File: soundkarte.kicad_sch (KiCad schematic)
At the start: 76 parts, among them J1 Data, J10 Address, J2 Control, J3 Bus Blaster, J4 Power, J5 1-28, J6 JTAG, J7 29-56, J8 Main Power, J9 Aux Power, U1 Teensy++2.0_(C)

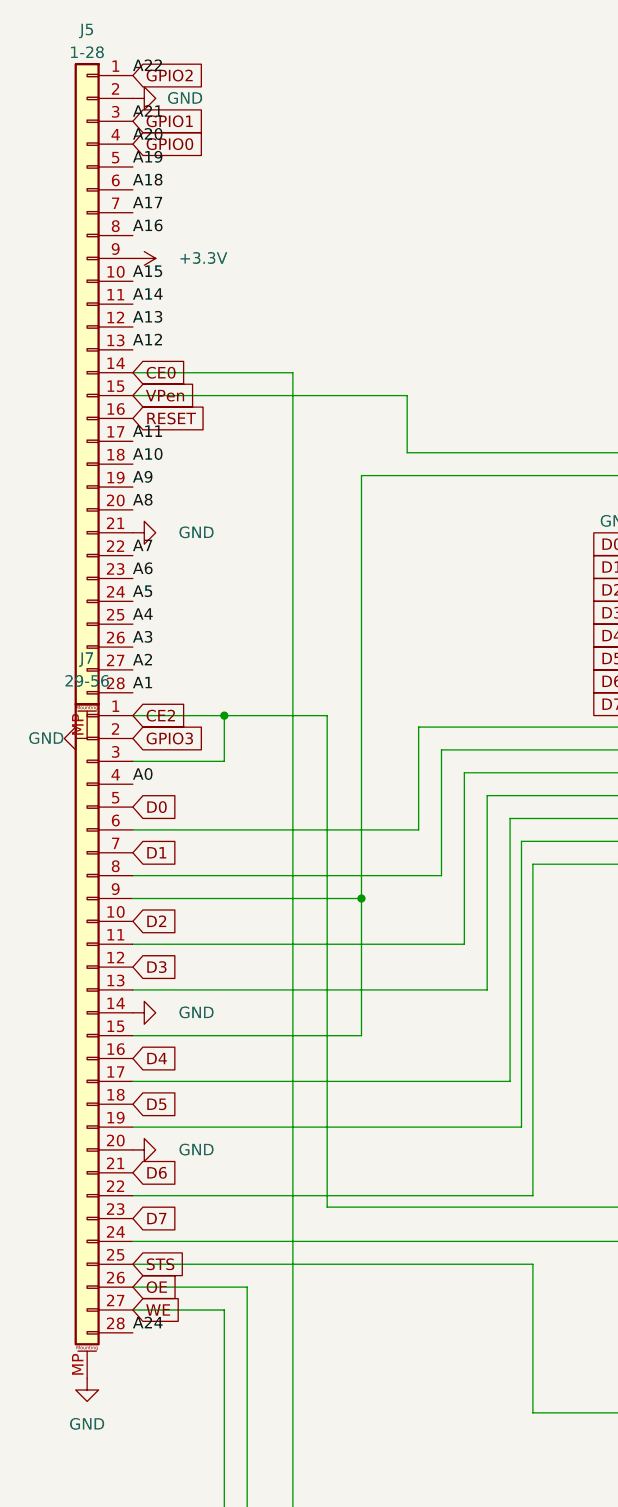
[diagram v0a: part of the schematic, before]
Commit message: 56pin sockel falls es geht geht es
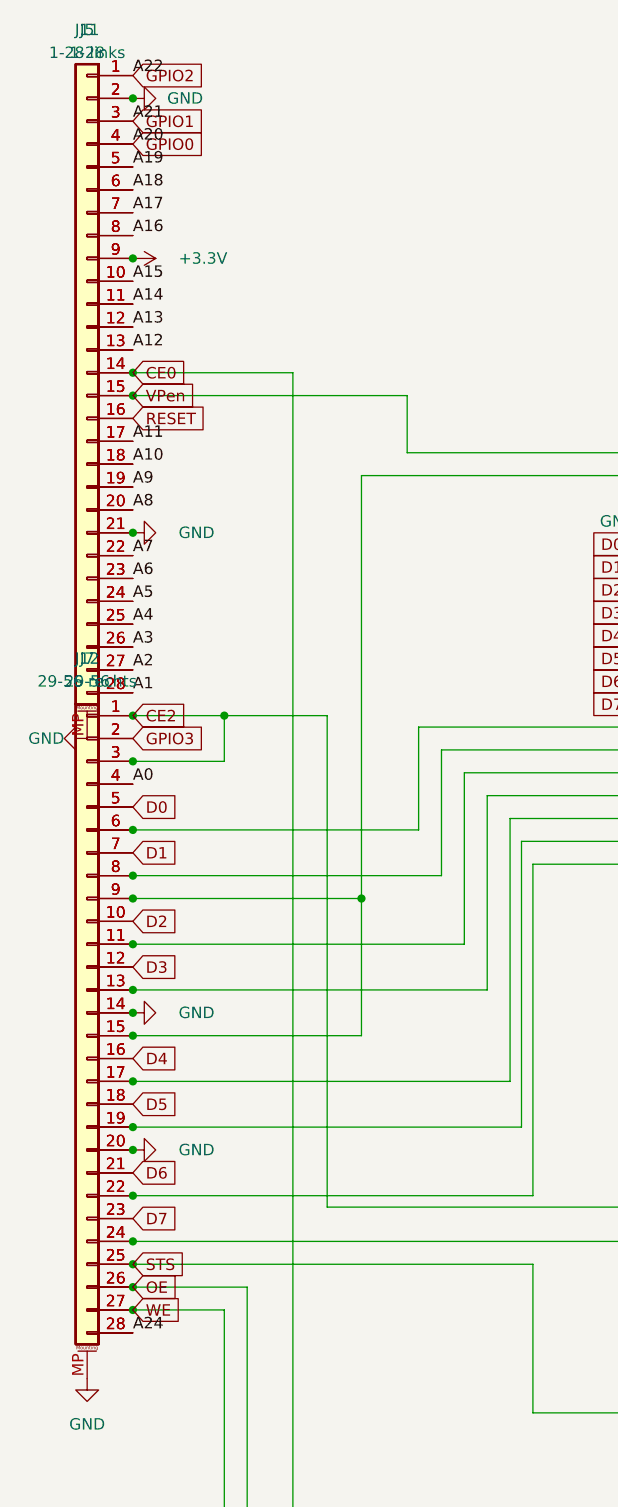
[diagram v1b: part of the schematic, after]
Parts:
- added J11: 1-28 links, Connector_PinHeader_2.54mm:PinHeader_1x28_P2.54mm_Vertical, symbol Connector_Generic:Conn_01x28
- added J12: 29-56 rechts, Connector_PinHeader_2.54mm:PinHeader_1x28_P2.54mm_Vertical, symbol Connector_Generic:Conn_01x28
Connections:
- net +3.3V: now also J11.9 (Pin_9)
- net A0: now also J12.4 (Pin_4)
- net A1: now also J11.28 (Pin_28)
- net A10: now also J11.18 (Pin_18)
- net A11: now also J11.17 (Pin_17)
- net A12: now also J11.13 (Pin_13)
- net A13: now also J11.12 (Pin_12)
- net A14: now also J11.11 (Pin_11)
- net A15: now also J11.10 (Pin_10)
- net A16: now also J11.8 (Pin_8)
- net A17: now also J11.7 (Pin_7)
- net A18: now also J11.6 (Pin_6)
- net A19: now also J11.5 (Pin_5)
- net A2: now also J11.27 (Pin_27)
- net A24: now also J12.28 (Pin_28)
- net A3: now also J11.26 (Pin_26)
- net A4: now also J11.25 (Pin_25)
- net A5: now also J11.24 (Pin_24)
- net A6: now also J11.23 (Pin_23)
- net A7: now also J11.22 (Pin_22)
- net A8: now also J11.20 (Pin_20)
- net A9: now also J11.19 (Pin_19)
- net CE0: now also J11.14 (Pin_14)
- net CE2: now also J12.1 (Pin_1), J12.3 (Pin_3)
- net D0: now also J12.5 (Pin_5)
- net D1: now also J12.7 (Pin_7)
- net D10: now also J12.11 (Pin_11)
- net D11: now also J12.13 (Pin_13)
- net D12: now also J12.17 (Pin_17)
- net D13: now also J12.19 (Pin_19)
- net D14: now also J12.22 (Pin_22)
- net D15: now also J12.24 (Pin_24)
- net D2: now also J12.10 (Pin_10)
- net D3: now also J12.12 (Pin_12)
- net D4: now also J12.16 (Pin_16)
- net D5: now also J12.18 (Pin_18)
- net D6: now also J12.21 (Pin_21)
- net D7: now also J12.23 (Pin_23)
- net D8: now also J12.6 (Pin_6)
- net D9: now also J12.8 (Pin_8)
- net GND: now also J11.2 (Pin_2), J11.21 (Pin_21), J12.14 (Pin_14), J12.20 (Pin_20)
- net GPIO0: now also J11.4 (Pin_4)
- net GPIO1: now also J11.3 (Pin_3)
- net GPIO2: now also J11.1 (Pin_1)
- net GPIO3: now also J12.2 (Pin_2)
- net OE: now also J12.26 (Pin_26)
- net RESET: now also J11.16 (Pin_16)
- net STS: now also J12.25 (Pin_25)
- net VPen: now also J11.15 (Pin_15)
- net WE: now also J12.27 (Pin_27)
- net at J4.8 (Pin_8), J7.15 (Pin_15), J7.9 (Pin_9): now also J12.15 (Pin_15), J12.9 (Pin_9)
